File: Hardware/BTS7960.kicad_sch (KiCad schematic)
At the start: 29 parts, among them J10 Screw_Terminal_01x04, J11 Screw_Terminal_01x04, J4 Screw_Terminal_01x04, U7 HCPL-2631, U8 HCPL-2631

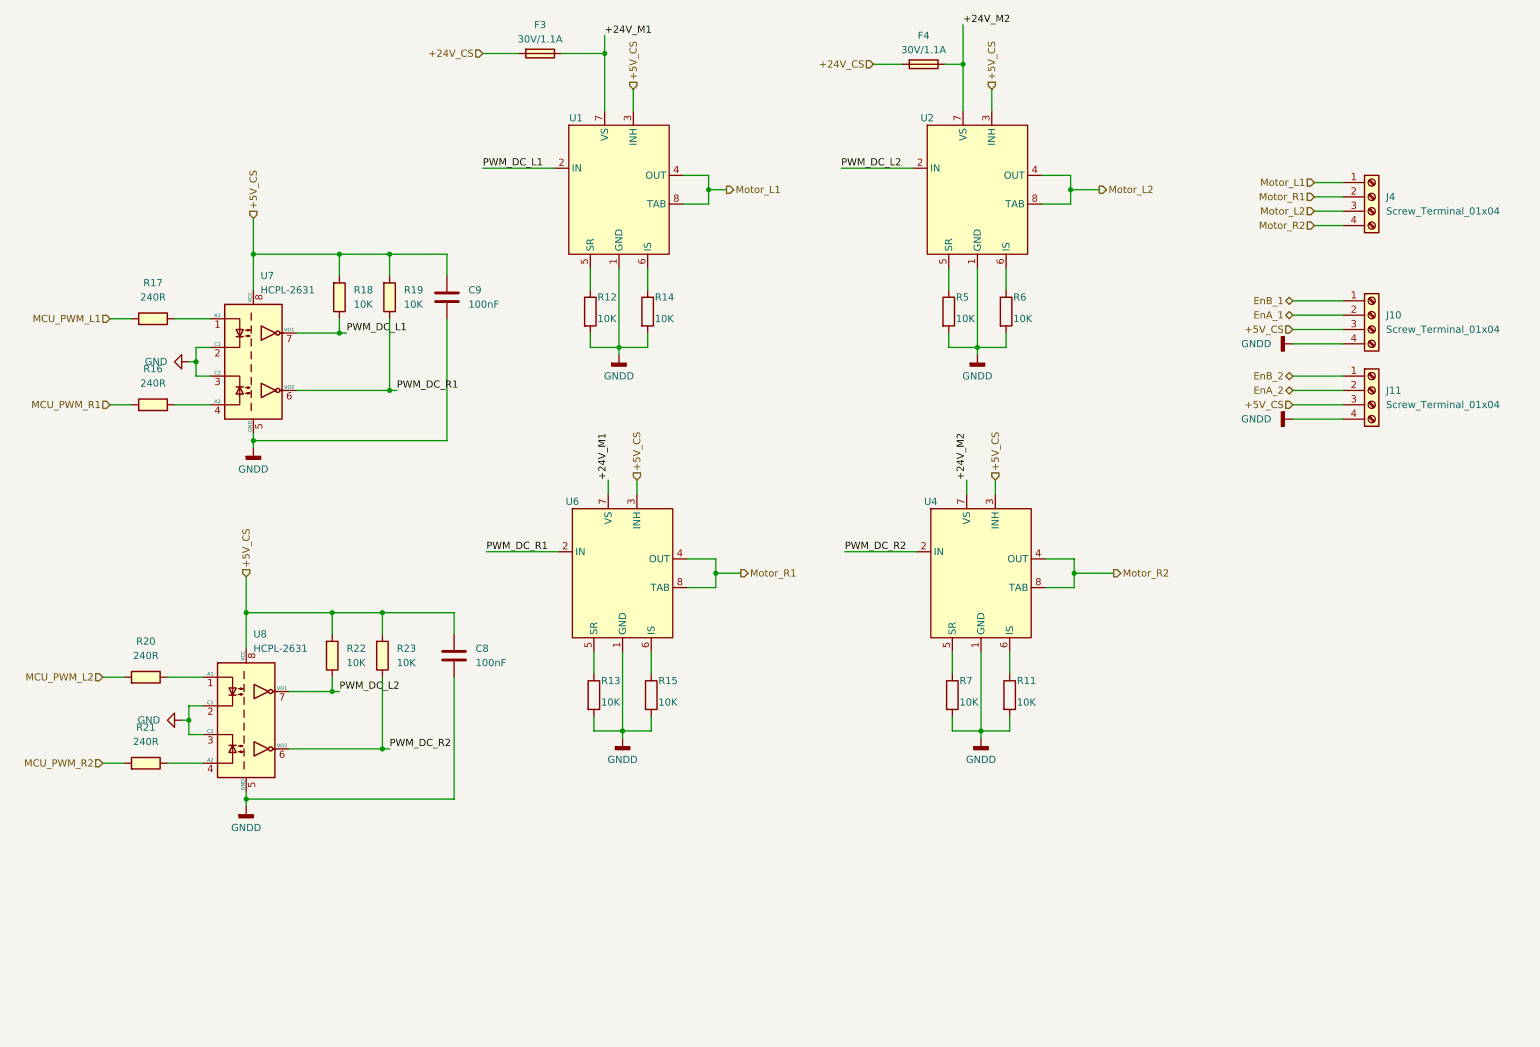
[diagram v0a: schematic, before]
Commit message: Add PCB
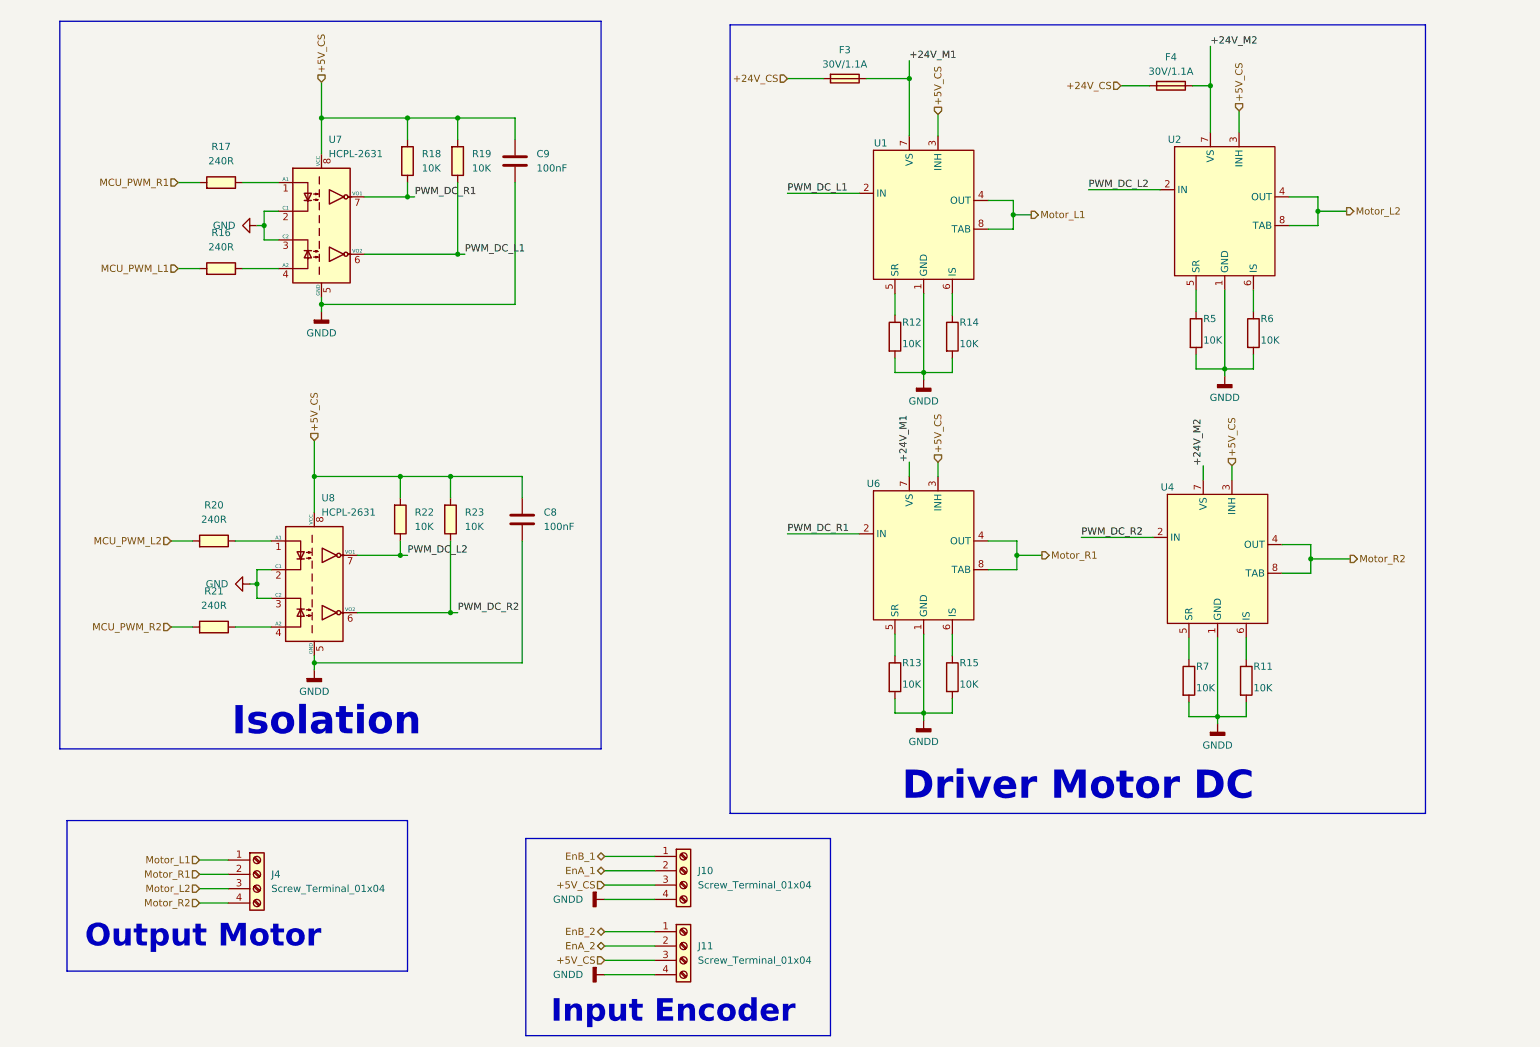
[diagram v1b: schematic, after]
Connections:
- net MCU_PWM_L1: now also R16.1; no longer R17.1
- net MCU_PWM_R1: now also R17.1; no longer R16.1
- net PWM_DC_L1: now also R19.2, U7.6 (VO2); no longer R18.2, U7.7 (VO1)
- net PWM_DC_R1: now also R18.2, U7.7 (VO1); no longer R19.2, U7.6 (VO2)
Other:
- note added: "Driver Motor DC"
- note added: "Input Encoder"
- note added: "Isolation"
- note added: "Output Motor"
- moved on the sheet: C8, C9, F3, F4, J10, J11, J4, R11, R12, R13, R14, R15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
